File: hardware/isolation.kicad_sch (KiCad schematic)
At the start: 8 parts, among them IC2 UCC12040DVER, IC3 MCP1700T-3302E_TT

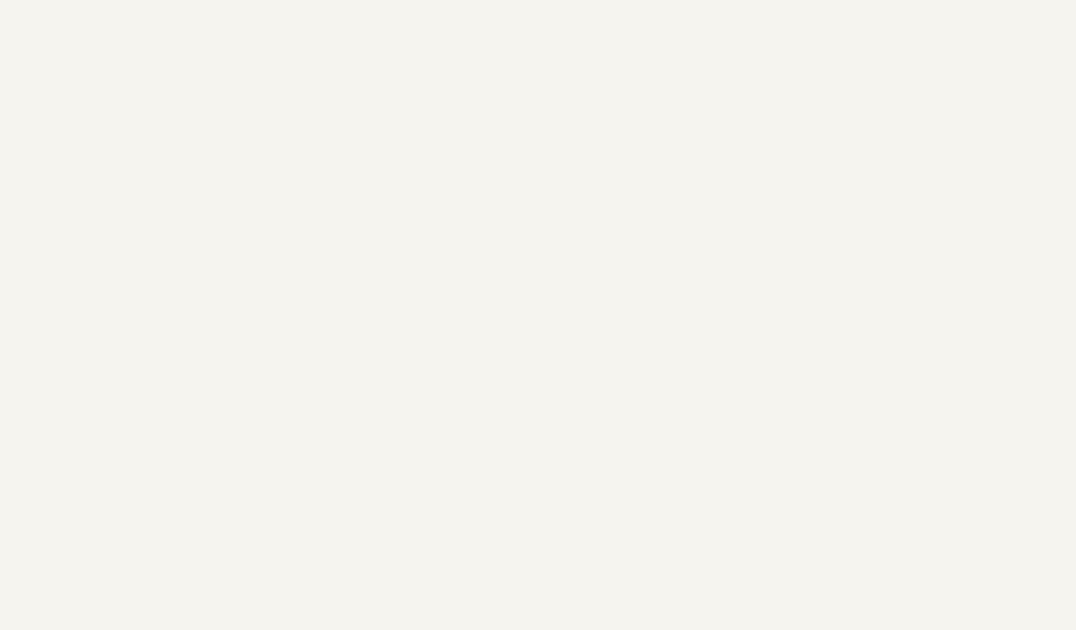
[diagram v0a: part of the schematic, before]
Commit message: Further ISO bridge development
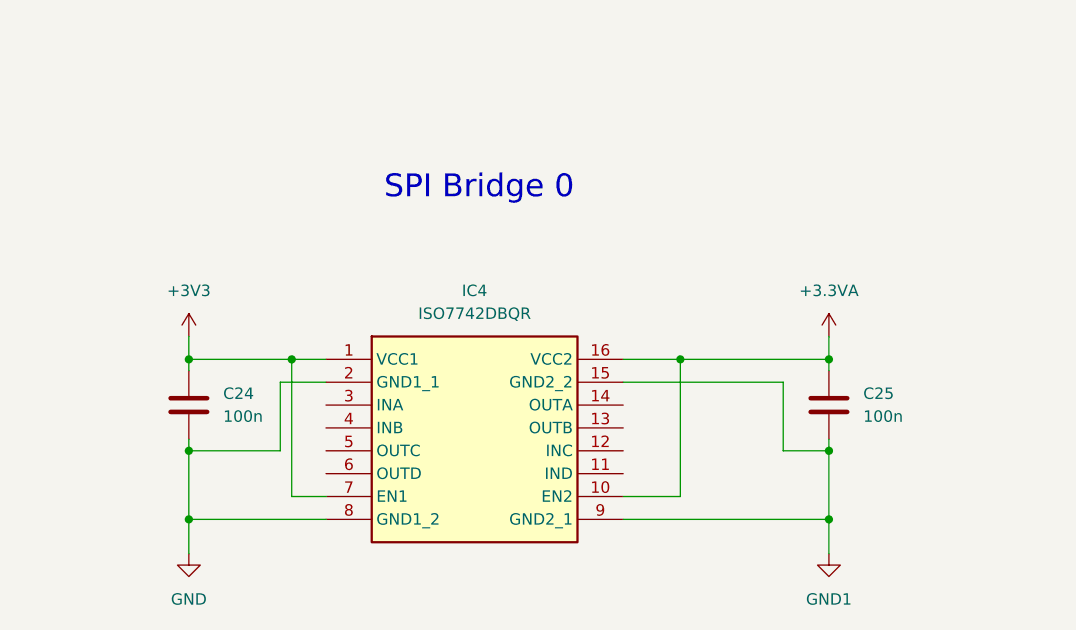
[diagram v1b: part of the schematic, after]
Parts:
- added C24, C25: 100n, Capacitor_SMD:C_0402_1005Metric, symbol Device:C
- added IC4: ISO7742DBQR, Stuttgart:SOP64P600X175-16N, symbol Stuttgart:ISO7742DBQR
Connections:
- net +3.3VA: now also C25.1, IC4.10 (EN2), IC4.16 (VCC2)
- net GND: now also C24.2, IC4.2 (GND1_1), IC4.8 (GND1_2)
- net GND1: now also C25.2, IC4.15 (GND2_2), IC4.9 (GND2_1)
- new net +3V3: C24.1, IC4.1 (VCC1), IC4.7 (EN1)
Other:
- note added: "SPI Bridge 0"
